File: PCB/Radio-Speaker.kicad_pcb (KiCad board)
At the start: 2 copper layers, 73.2 x 32.9 mm, 21 parts, among them CN1 PJ-3200, J1 R_SPK, J2 L_SPK, SW1 SW_Push, U1 RDA5807MRRD-102V2.0, U2 XIAO-RP2040-DIP, U3 TDA2822NBD, U4 m18

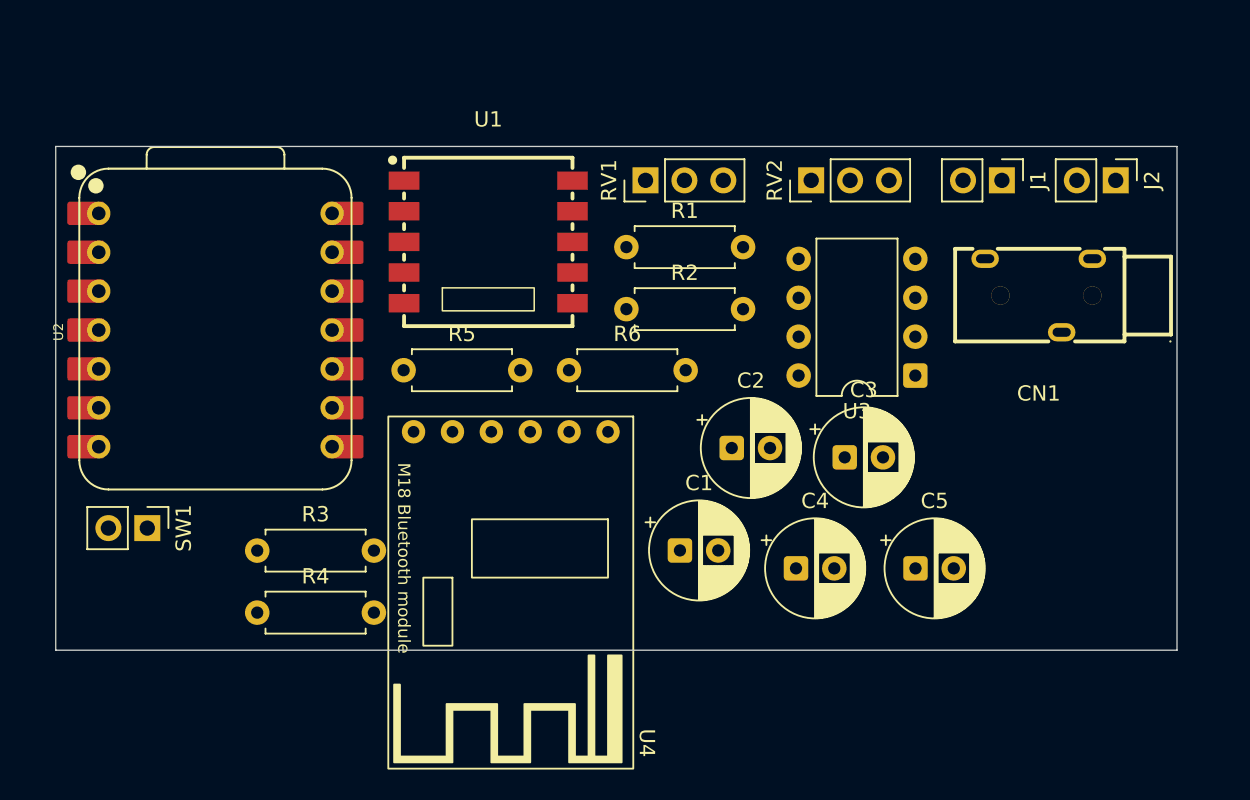
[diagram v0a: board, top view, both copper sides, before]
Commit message: LOTS of new stuff
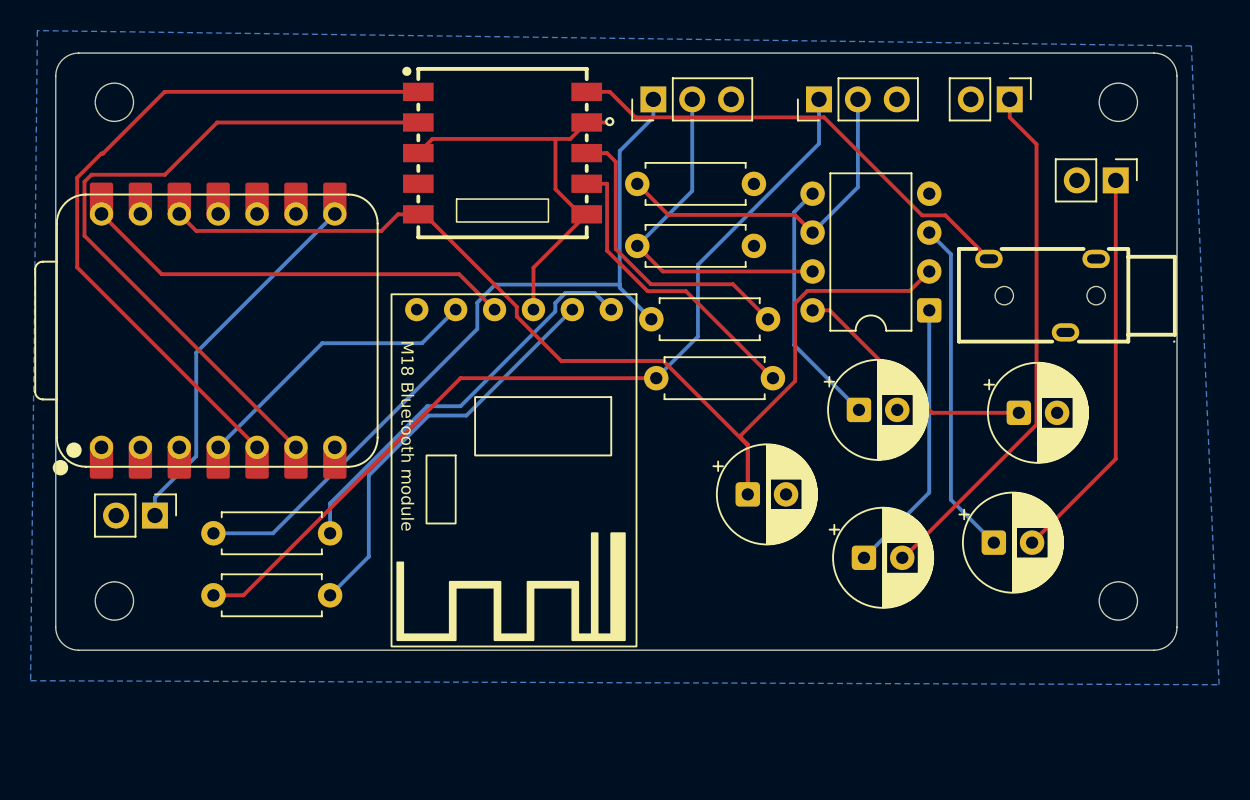
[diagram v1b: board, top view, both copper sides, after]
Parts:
- added H1: MountingHole, MountingHole:MountingHole_2.5mm, F.Cu at (90.7, 53.2)
- added H2: MountingHole, MountingHole:MountingHole_2.5mm, F.Cu at (156.2, 53.2)
- added H3: MountingHole, MountingHole:MountingHole_2.5mm, F.Cu at (90.7, 85.8)
- added H4: MountingHole, MountingHole:MountingHole_2.5mm, F.Cu at (156.2, 85.8)
- moved R5 16.5 mm to (125.7, 67.4)
- moved C3 11.7 mm to (149.7, 73.5)
- moved C2 8.68 mm to (139.3, 73.3)
- moved U4 7.98 mm to (116.8, 66.8)
- moved U1 5.87 mm to (116.0, 56.6)
- moved C1 5.75 mm to (132.0, 78.8)
- moved R6 5.72 mm to (126.0, 71.3)
- moved C5 5.39 mm to (148.1, 82.0)
- moved RV2 5.31 mm to (136.7, 53.0)
- moved RV1 5.31 mm to (125.9, 53.0)
- moved J1 5.31 mm to (149.1, 53.0)
- moved C4 4.49 mm to (139.6, 83.0)
- moved U3 4.36 mm to (143.9, 66.8)
- moved R1 4.19 mm to (124.8, 58.6)
- moved R2 4.19 mm to (124.8, 62.6)
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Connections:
- C1 pad 1: VCC -> +3V3
- U2 pad 14: unconnected-(U2-VBUS-Pad14) -> +5V
- U3 pad 2: VCC -> +3V3
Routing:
- net +3V3: track 0.00 -> 72.5 mm
- net L_MIX: track 0.00 -> 57.4 mm
- net R_MIX: track 0.00 -> 50.4 mm
- net SDA: track 0.00 -> 47.9 mm
- net SCL: track 0.00 -> 47.3 mm
- net R_AMP_OUT: track 0.00 -> 34.3 mm
- net Net-(U1-ANT): track 0.00 -> 30.8 mm
- net +5V: track 0.00 -> 29.1 mm
- net GND: track 0.00 -> 27.9 mm, vias 0 -> 1
- net Net-(U4-R): track 0.00 -> 26.8 mm
- net Net-(U4-L): track 0.00 -> 26.7 mm
- net L_AMP_OUT: track 0.00 -> 25.9 mm
- net Net-(U2-P1_D7_RX): track 0.00 -> 25.4 mm
- net Net-(U3-IN1): track 0.00 -> 23.2 mm
- net Net-(U3-IN2): track 0.00 -> 22.7 mm
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- added copper zone on B.Cu, net GND
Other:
- board size 73.2 x 32.9 mm -> 73.2 x 39 mm
